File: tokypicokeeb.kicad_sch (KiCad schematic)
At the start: 41 parts, among them SW1 SW_Push, U1 PicoW

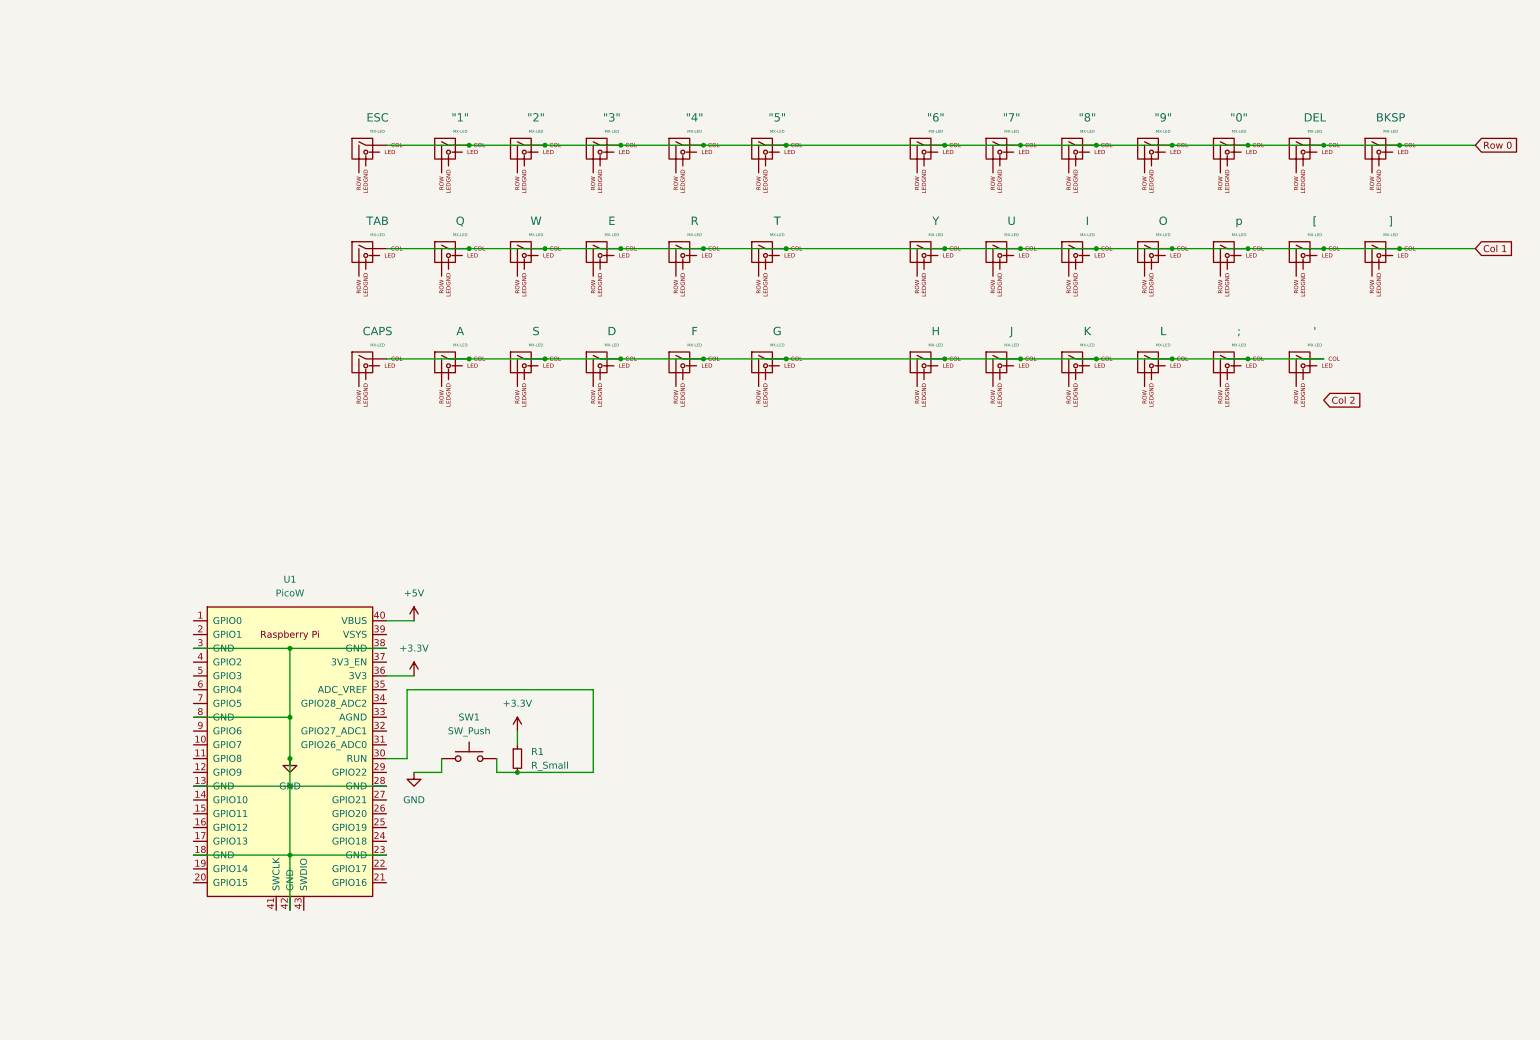
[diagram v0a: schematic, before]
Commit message: updated matrix
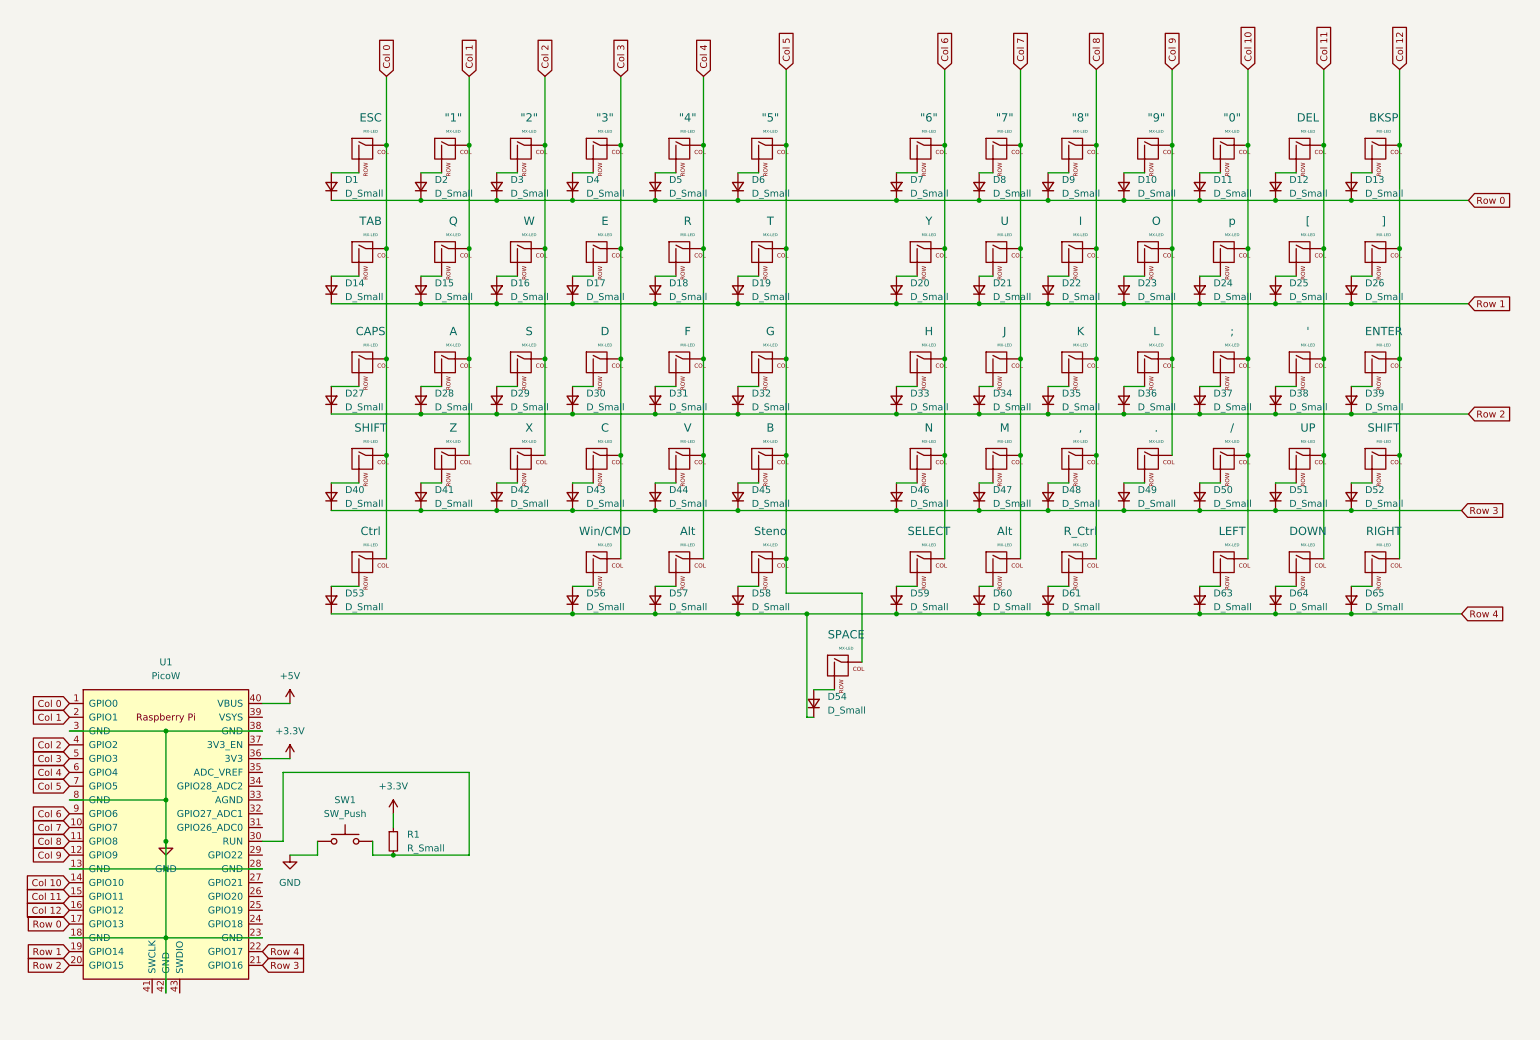
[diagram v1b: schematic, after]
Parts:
- added ,, ., /, Alt (x2), B, C, Ctrl, DOWN, ENTER, LEFT, M, N, RIGHT, R_Ctrl, SELECT, SHIFT (x2), SPACE, Steno, UP, V, Win/CMD, X, Z: MX-LED, symbol MX_Alps_Hybrid:MX-NoLED
- added D1, D10, D11, D12, D13, D14, D15, D16, D17, D18, D19, D2, D20, D21, D22, D23, D24, D25, D26, D27, D28, D29, D3, D30, D31, D32, D33, D34, D35, D36, D37, D38, D39, D4, D40, D41, D42, D43, D44, D45, D46, D47, D48, D49, D5, D50, D51, D52, D53, D54, D56, D57, D58, D59, D6, D60, D61, D63, D64, D65, D7, D8, D9: D_Small, symbol Device:D_Small
- "0", "1", "2", "3", "4", "5", "6", "7", "8", "9", ', ;, A, BKSP, CAPS, D, DEL, E, ESC, F, G, H, I, J, K, L, O, Q, R, S, T, TAB, U, W, Y, [, ], p: symbol MX_Alps_Hybrid:MX-LED -> MX_Alps_Hybrid:MX-NoLED
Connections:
- net Col 1: now also "1".1 (COL), A.1 (COL), U1.2 (GPIO1), Z.1 (COL); no longer E.1 (COL), I.1 (COL), O.1 (COL), R.1 (COL), T.1 (COL), TAB.1 (COL), U.1 (COL), W.1 (COL), Y.1 (COL), [.1 (COL), ].1 (COL), p.1 (COL)
- net Col 2: now also "2".1 (COL), S.1 (COL), U1.4 (GPIO2), W.1 (COL), X.1 (COL)
- net Row 0: now also U1.17 (GPIO13), D1.1 (K), D10.1 (K), D11.1 (K), D12.1 (K), D13.1 (K), D2.1 (K), D3.1 (K), D4.1 (K), D5.1 (K), D6.1 (K), D7.1 (K), D8.1 (K), D9.1 (K); no longer "0".1 (COL), "1".1 (COL), "2".1 (COL), "3".1 (COL), "4".1 (COL), "5".1 (COL), "6".1 (COL), "7".1 (COL), "8".1 (COL), "9".1 (COL), BKSP.1 (COL), DEL.1 (COL), ESC.1 (COL)
- net at R.2 (ROW): now also D18.2 (A)
- net at A.2 (ROW): now also D28.2 (A)
- net at I.2 (ROW): now also D22.2 (A)
- net at G.2 (ROW): now also D32.2 (A)
- net at U.2 (ROW): now also D21.2 (A)
- net at Y.2 (ROW): now also D20.2 (A)
- net at "5".2 (ROW): now also D6.2 (A)
- net at W.2 (ROW): now also D16.2 (A)
- net at "0".2 (ROW): now also D11.2 (A)
- net at Q.2 (ROW): now also D15.2 (A)
- net at ESC.2 (ROW): now also D1.2 (A)
- net at "8".2 (ROW): now also D9.2 (A)
- net at "2".2 (ROW): now also D3.2 (A)
- net at "7".2 (ROW): now also D8.2 (A)
- net at L.2 (ROW): now also D36.2 (A)
- net at T.2 (ROW): now also D19.2 (A)
- net at K.2 (ROW): now also D35.2 (A)
- net at p.2 (ROW): now also D24.2 (A)
- net at O.2 (ROW): now also D23.2 (A)
- net at J.2 (ROW): now also D34.2 (A)
- net at S.2 (ROW): now also D29.2 (A)
- net at D.2 (ROW): now also D30.2 (A)
- net at DEL.2 (ROW): now also D12.2 (A)
- net at CAPS.2 (ROW): now also D27.2 (A)
- net at F.2 (ROW): now also D31.2 (A)
- net at '.2 (ROW): now also D38.2 (A)
- net at TAB.2 (ROW): now also D14.2 (A)
- net at H.2 (ROW): now also D33.2 (A)
- net Col 0: now reaches U1.1 (GPIO0)
- net Col 0: now also CAPS.1 (COL), ESC.1 (COL), TAB.1 (COL), Ctrl.1 (COL), SHIFT.1 (COL)
- net Col 7: now reaches U1.10 (GPIO7)
- net Col 7: now also "7".1 (COL), J.1 (COL), U.1 (COL), Alt.1 (COL), M.1 (COL)
- net Col 8: now reaches U1.11 (GPIO8)
- net Col 8: now also "8".1 (COL), I.1 (COL), K.1 (COL), ,.1 (COL), R_Ctrl.1 (COL)
- net Col 9: now reaches U1.12 (GPIO9)
- net Col 9: now also "9".1 (COL), L.1 (COL), O.1 (COL), ..1 (COL)
- net Col 10: now reaches U1.14 (GPIO10)
- net Col 10: now also "0".1 (COL), ;.1 (COL), p.1 (COL), /.1 (COL), LEFT.1 (COL)
- net Col 11: now reaches U1.15 (GPIO11)
- net Col 11: now also '.1 (COL), DEL.1 (COL), [.1 (COL), DOWN.1 (COL), UP.1 (COL)
- net Col 12: now reaches U1.16 (GPIO12)
- net Col 12: now also BKSP.1 (COL), ].1 (COL), ENTER.1 (COL), RIGHT.1 (COL), SHIFT.1 (COL)
- net Row 1: now reaches U1.19 (GPIO14)
- net Row 1: now also D14.1 (K), D15.1 (K), D16.1 (K), D17.1 (K), D18.1 (K), D19.1 (K), D20.1 (K), D21.1 (K), D22.1 (K), D23.1 (K), D24.1 (K), D25.1 (K), D26.1 (K)
- net Row 2: now reaches U1.20 (GPIO15)
- net Row 2: now also D27.1 (K), D28.1 (K), D29.1 (K), D30.1 (K), D31.1 (K), D32.1 (K), D33.1 (K), D34.1 (K), D35.1 (K), D36.1 (K), D37.1 (K), D38.1 (K), D39.1 (K)
- net Row 3: now reaches U1.21 (GPIO16)
- net Row 3: now also D40.1 (K), D41.1 (K), D42.1 (K), D43.1 (K), D44.1 (K), D45.1 (K), D46.1 (K), D47.1 (K), D48.1 (K), D49.1 (K), D50.1 (K), D51.1 (K), D52.1 (K)
- net Row 4: now reaches U1.22 (GPIO17)
- net Row 4: now also D53.1 (K), D54.1 (K), D56.1 (K), D57.1 (K), D58.1 (K), D59.1 (K), D60.1 (K), D61.1 (K), D63.1 (K), D64.1 (K), D65.1 (K)
- net Col 3: now reaches U1.5 (GPIO3)
- net Col 3: now also "3".1 (COL), D.1 (COL), E.1 (COL), C.1 (COL), Win/CMD.1 (COL)
- net Col 4: now reaches U1.6 (GPIO4)
- net Col 4: now also "4".1 (COL), F.1 (COL), R.1 (COL), Alt.1 (COL), V.1 (COL)
- net Col 5: now reaches U1.7 (GPIO5)
- net Col 5: now also "5".1 (COL), G.1 (COL), T.1 (COL), B.1 (COL), SPACE.1 (COL), Steno.1 (COL)
- net Col 6: now reaches U1.9 (GPIO6)
- net Col 6: now also "6".1 (COL), H.1 (COL), Y.1 (COL), N.1 (COL), SELECT.1 (COL)
- net at "3".2 (ROW): now also D4.2 (A)
- net at BKSP.2 (ROW): now also D13.2 (A)
- net at "1".2 (ROW): now also D2.2 (A)
- net at [.2 (ROW): now also D25.2 (A)
- net at E.2 (ROW): now also D17.2 (A)
- net at ;.2 (ROW): now also D37.2 (A)
- net at "9".2 (ROW): now also D10.2 (A)
- net at "6".2 (ROW): now also D7.2 (A)
- net at ].2 (ROW): now also D26.2 (A)
- net at "4".2 (ROW): now also D5.2 (A)
- new net: D61.2 (A), R_Ctrl.2 (ROW)
- new net: /.2 (ROW), D50.2 (A)
- new net: B.2 (ROW), D45.2 (A)
- new net: D52.2 (A), SHIFT.2 (ROW)
- new net: D39.2 (A), ENTER.2 (ROW)
- new net: D58.2 (A), Steno.2 (ROW)
- new net: Alt.2 (ROW), D57.2 (A)
- new net: D51.2 (A), UP.2 (ROW)
- new net: D40.2 (A), SHIFT.2 (ROW)
- new net: D46.2 (A), N.2 (ROW)
- new net: D56.2 (A), Win/CMD.2 (ROW)
- new net: Alt.2 (ROW), D60.2 (A)
- new net: D64.2 (A), DOWN.2 (ROW)
- new net: ..2 (ROW), D49.2 (A)
- new net: D63.2 (A), LEFT.2 (ROW)
- new net: D41.2 (A), Z.2 (ROW)
- new net: D47.2 (A), M.2 (ROW)
- new net: D59.2 (A), SELECT.2 (ROW)
- new net: D44.2 (A), V.2 (ROW)
- new net: C.2 (ROW), D43.2 (A)
- new net: D65.2 (A), RIGHT.2 (ROW)
- new net: Ctrl.2 (ROW), D53.2 (A)
- new net: ,.2 (ROW), D48.2 (A)
- new net: D54.2 (A), SPACE.2 (ROW)
- new net: D42.2 (A), X.2 (ROW)
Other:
- moved on the sheet: R1, SW1, U1

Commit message: re-organized things
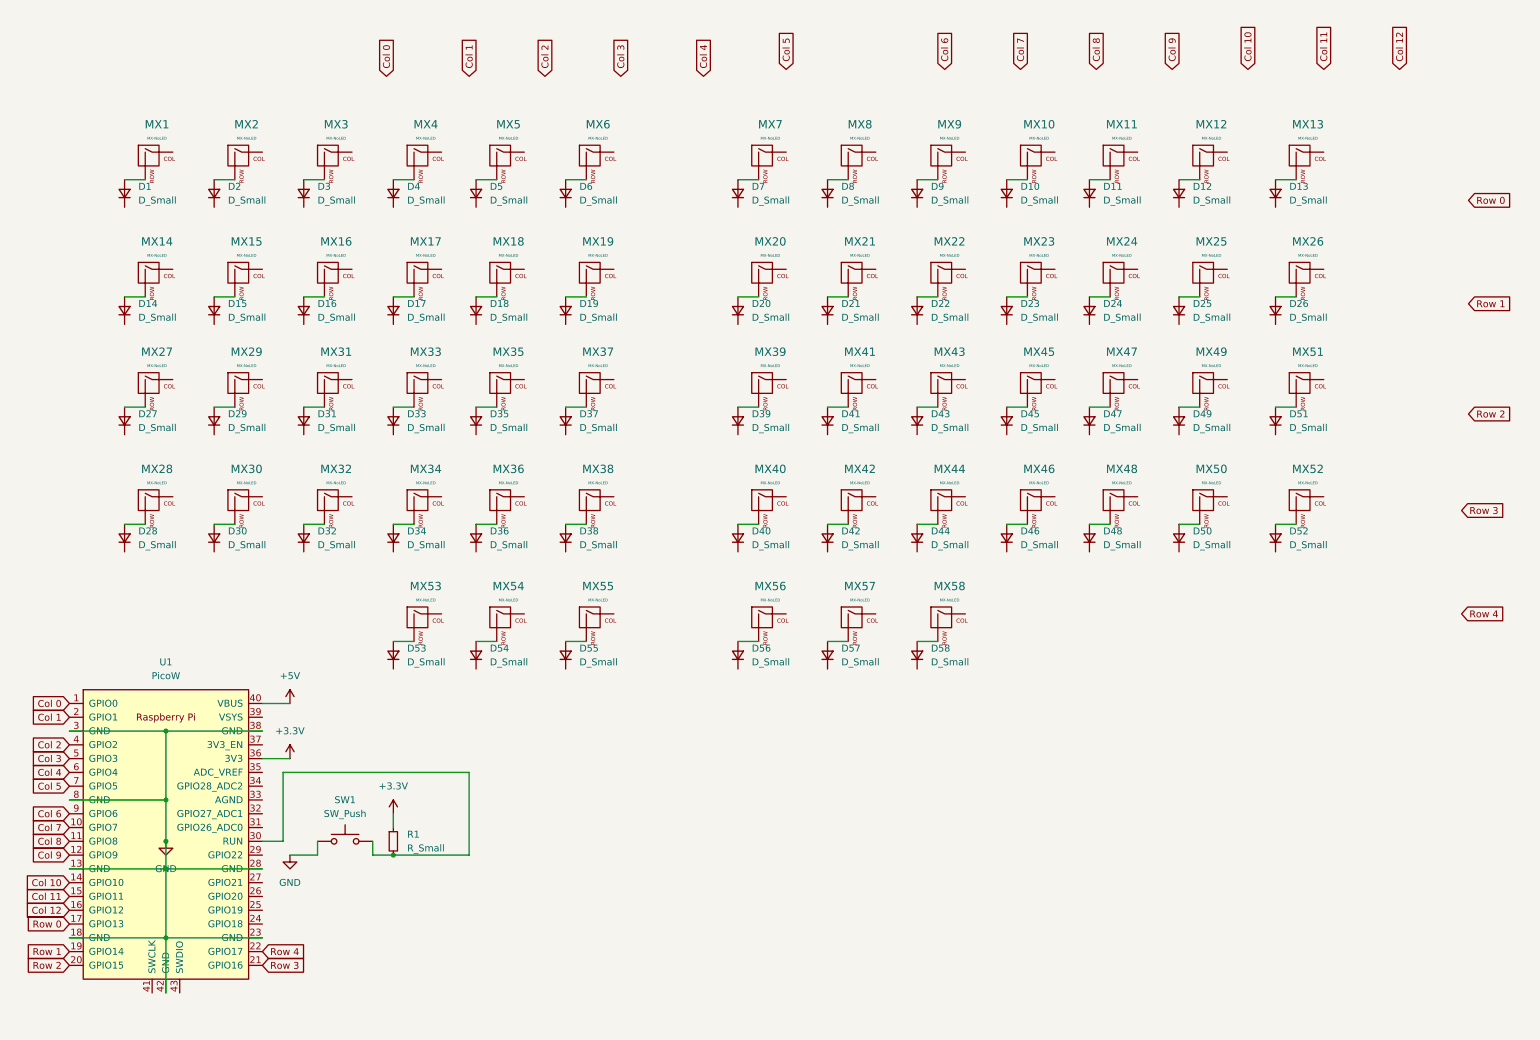
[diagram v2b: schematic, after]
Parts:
- removed "0", "1", "2", "3", "4", "5", "6", "7", "8", "9", ', ,, ., /, ;, A, Alt (x2), B, BKSP, C, CAPS, Ctrl, D, DEL, DOWN, E, ENTER, ESC, F, G, H, I, J, K, L, LEFT, M, N, O, Q, R, RIGHT, R_Ctrl, S, SELECT, SHIFT (x2), SPACE, Steno, T, TAB, U, UP, V, W, Win/CMD, X, Y, Z, [, ], p: MX-LED, symbol MX_Alps_Hybrid:MX-NoLED
- removed D59, D60, D61, D63, D64, D65: D_Small, symbol Device:D_Small
- added D55: D_Small, symbol Device:D_Small
- added MX1, MX10, MX11, MX12, MX13, MX14, MX15, MX16, MX17, MX18, MX19, MX2, MX20, MX21, MX22, MX23, MX24, MX25, MX26, MX27, MX28, MX29, MX3, MX30, MX31, MX32, MX33, MX34, MX35, MX36, MX37, MX38, MX39, MX4, MX40, MX41, MX42, MX43, MX44, MX45, MX46, MX47, MX48, MX49, MX5, MX50, MX51, MX52, MX53, MX54, MX55, MX56, MX57, MX58, MX6, MX7, MX8, MX9: MX-NoLED, symbol MX_Alps_Hybrid:MX-NoLED
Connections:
- net Row 0: no longer D1.1 (K), D10.1 (K), D11.1 (K), D12.1 (K), D13.1 (K), D2.1 (K), D3.1 (K), D4.1 (K), D5.1 (K), D6.1 (K), D7.1 (K), D8.1 (K), D9.1 (K)
- net Row 1: no longer D14.1 (K), D15.1 (K), D16.1 (K), D17.1 (K), D18.1 (K), D19.1 (K), D20.1 (K), D21.1 (K), D22.1 (K), D23.1 (K), D24.1 (K), D25.1 (K), D26.1 (K)
- net Row 2: no longer D27.1 (K), D28.1 (K), D29.1 (K), D30.1 (K), D31.1 (K), D32.1 (K), D33.1 (K), D34.1 (K), D35.1 (K), D36.1 (K), D37.1 (K), D38.1 (K), D39.1 (K)
- net Row 3: no longer D40.1 (K), D41.1 (K), D42.1 (K), D43.1 (K), D44.1 (K), D45.1 (K), D46.1 (K), D47.1 (K), D48.1 (K), D49.1 (K), D50.1 (K), D51.1 (K), D52.1 (K)
- net Row 4: no longer D53.1 (K), D54.1 (K), D56.1 (K), D57.1 (K), D58.1 (K)
- net at D18.2 (A): now also MX18.2 (ROW)
- net at D28.2 (A): now also MX28.2 (ROW)
- net at D50.2 (A): now also MX50.2 (ROW)
- net at D45.2 (A): now also MX45.2 (ROW)
- net at D27.2 (A): now also MX27.2 (ROW)
- net at D36.2 (A): now also MX36.2 (ROW)
- net at D22.2 (A): now also MX22.2 (ROW)
- net at D32.2 (A): now also MX32.2 (ROW)
- net at D52.2 (A): now also MX52.2 (ROW)
- net at D21.2 (A): now also MX21.2 (ROW)
- net at D20.2 (A): now also MX20.2 (ROW)
- net at D6.2 (A): now also MX6.2 (ROW)
- net at D16.2 (A): now also MX16.2 (ROW)
- net at D3.2 (A): now also MX3.2 (ROW)
- net at D39.2 (A): now also MX39.2 (ROW)
- net at D11.2 (A): now also MX11.2 (ROW)
- net at D15.2 (A): now also MX15.2 (ROW)
- net at D58.2 (A): now also MX58.2 (ROW)
- net at D1.2 (A): now also MX1.2 (ROW)
- net at D30.2 (A): now also MX30.2 (ROW)
- net at D23.2 (A): now also MX23.2 (ROW)
- net at D57.2 (A): now also MX57.2 (ROW)
- net at D9.2 (A): now also MX9.2 (ROW)
- net at D10.2 (A): now also MX10.2 (ROW)
- net at D51.2 (A): now also MX51.2 (ROW)
- net at D40.2 (A): now also MX40.2 (ROW)
- net at D37.2 (A): now also MX37.2 (ROW)
- net at D46.2 (A): now also MX46.2 (ROW)
- net at D8.2 (A): now also MX8.2 (ROW)
- net at D34.2 (A): now also MX34.2 (ROW)
- net at D5.2 (A): now also MX5.2 (ROW)
- net at D26.2 (A): now also MX26.2 (ROW)
- net at D56.2 (A): now also MX56.2 (ROW)
- net at D19.2 (A): now also MX19.2 (ROW)
- net at D17.2 (A): now also MX17.2 (ROW)
- net at D35.2 (A): now also MX35.2 (ROW)
- net at D24.2 (A): now also MX24.2 (ROW)
- net at D29.2 (A): now also MX29.2 (ROW)
- net at D49.2 (A): now also MX49.2 (ROW)
- net at D33.2 (A): now also MX33.2 (ROW)
- net at D12.2 (A): now also MX12.2 (ROW)
- net at D41.2 (A): now also MX41.2 (ROW)
- net at D47.2 (A): now also MX47.2 (ROW)
- net at D38.2 (A): now also MX38.2 (ROW)
- net at D4.2 (A): now also MX4.2 (ROW)
- net at D44.2 (A): now also MX44.2 (ROW)
- net at D31.2 (A): now also MX31.2 (ROW)
- net at D25.2 (A): now also MX25.2 (ROW)
- net at D43.2 (A): now also MX43.2 (ROW)
- net at D14.2 (A): now also MX14.2 (ROW)
- net at D53.2 (A): now also MX53.2 (ROW)
- net at D48.2 (A): now also MX48.2 (ROW)
- net at D54.2 (A): now also MX54.2 (ROW)
- net at D13.2 (A): now also MX13.2 (ROW)
- net at D42.2 (A): now also MX42.2 (ROW)
- net at D2.2 (A): now also MX2.2 (ROW)
- net at D7.2 (A): now also MX7.2 (ROW)
- new net: D55.2 (A), MX55.2 (ROW)
